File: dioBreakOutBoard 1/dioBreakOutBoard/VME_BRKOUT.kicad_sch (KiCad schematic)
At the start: 2 parts, among them J11 56509455, J12 56509455

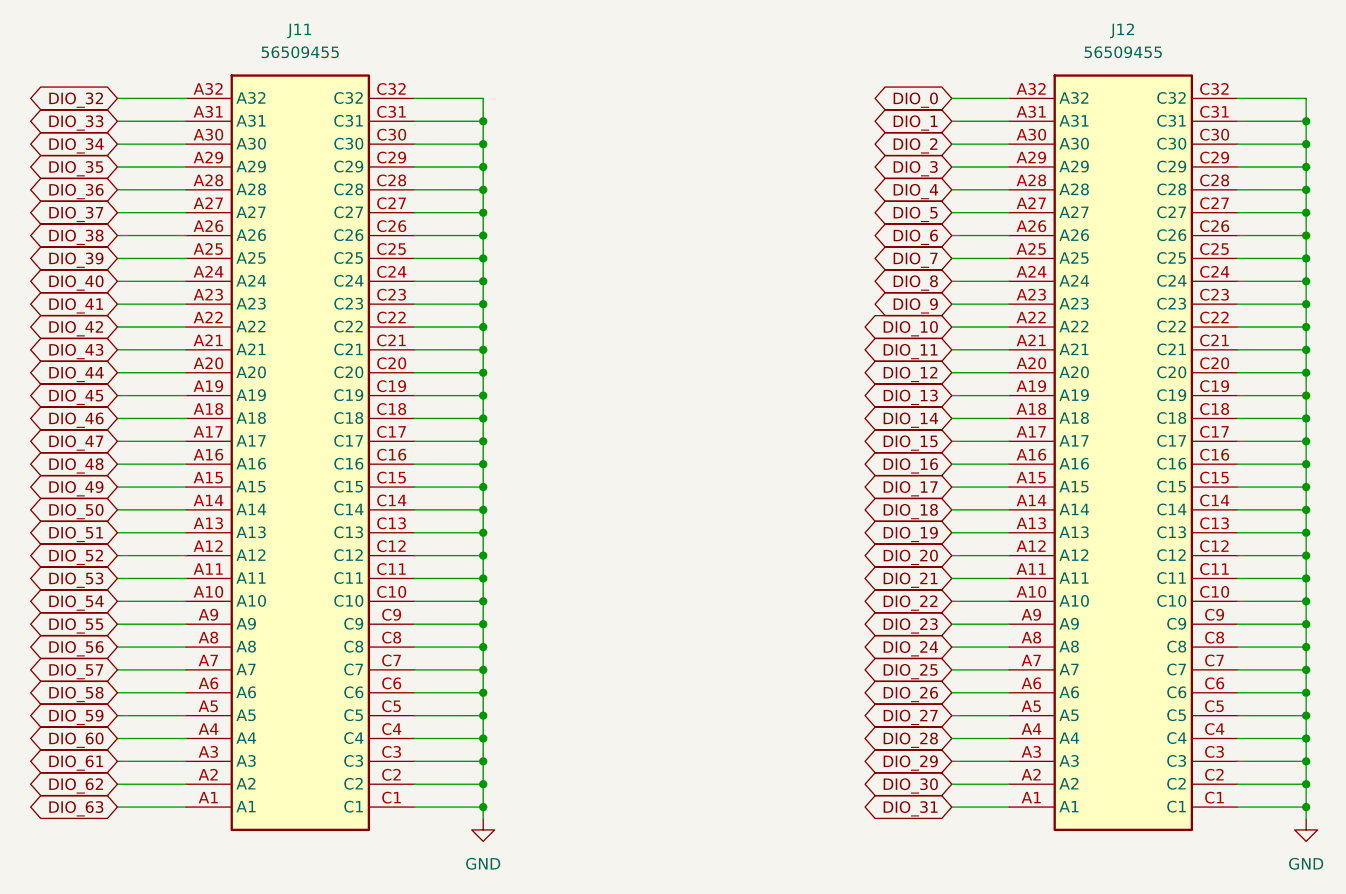
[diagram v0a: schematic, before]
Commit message: C:\Users\khernandez\KiCad\KiCad-Projects# Please enter the commit message for your changes. Lines starting
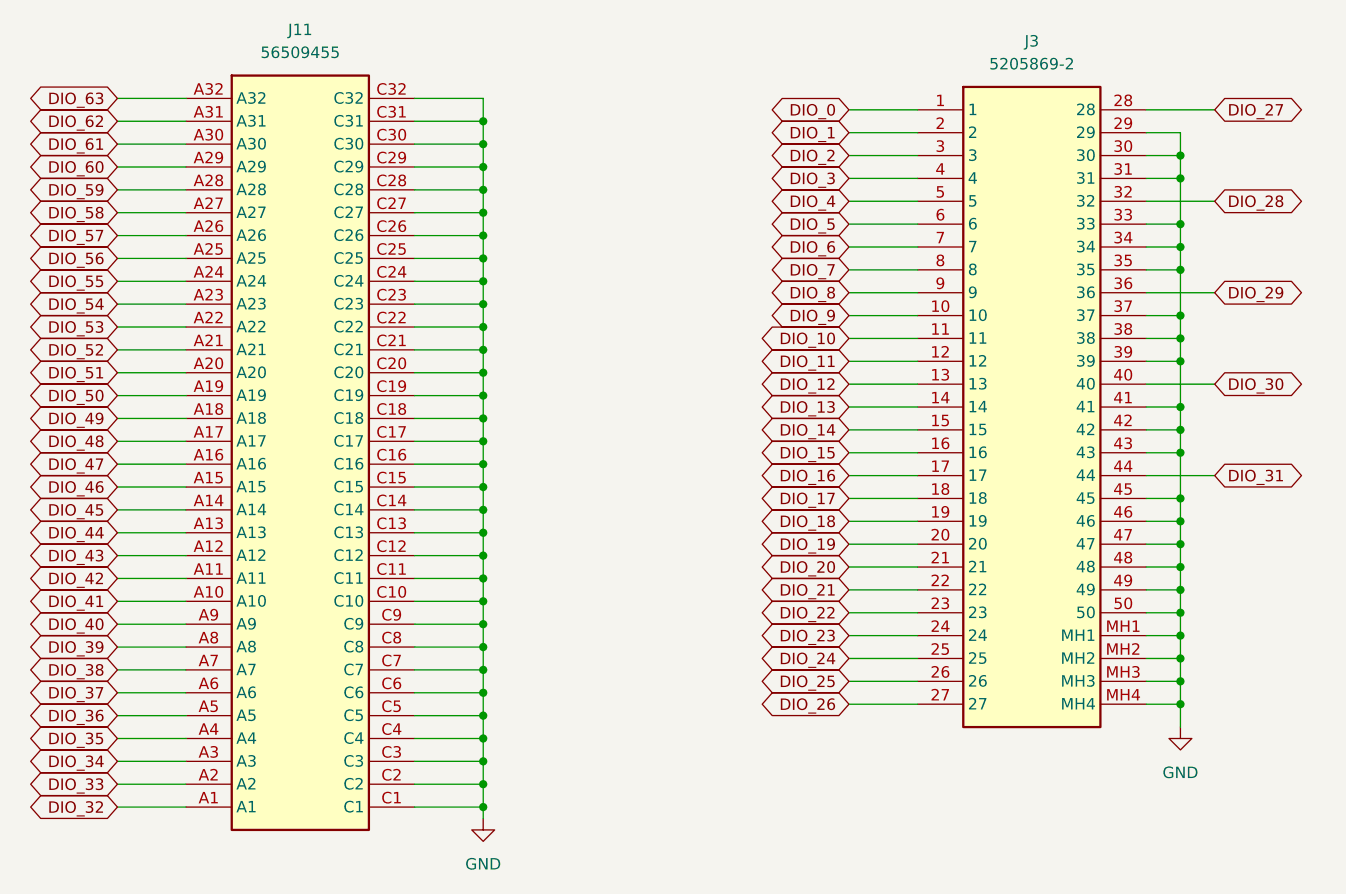
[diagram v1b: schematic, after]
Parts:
- removed J12: 56509455, Connectors_kmh:56509455, symbol 09031646922:09031646922
- added J3: 5205869-2, Connectors_kmh:52058692, symbol 5205869-2:5205869-2
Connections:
- net DIO_0: now also J3.1
- net DIO_1: now also J3.2
- net DIO_10: now also J3.11
- net DIO_11: now also J3.12
- net DIO_12: now also J3.13
- net DIO_13: now also J3.14
- net DIO_14: now also J3.15
- net DIO_15: now also J3.16
- net DIO_16: now also J3.17
- net DIO_17: now also J3.18
- net DIO_18: now also J3.19
- net DIO_19: now also J3.20
- net DIO_2: now also J3.3
- net DIO_20: now also J3.21
- net DIO_21: now also J3.22
- net DIO_22: now also J3.23
- net DIO_23: now also J3.24
- net DIO_24: now also J3.25
- net DIO_25: now also J3.26
- net DIO_26: now also J3.27
- net DIO_27: now also J3.28
- net DIO_28: now also J3.32
- net DIO_29: now also J3.36
- net DIO_3: now also J3.4
- net DIO_30: now also J3.40
- net DIO_31: now also J3.44
- net DIO_32: now also J11.A1; no longer J11.A32
- net DIO_33: now also J11.A2; no longer J11.A31
- net DIO_34: now also J11.A3; no longer J11.A30
- net DIO_35: now also J11.A4; no longer J11.A29
- net DIO_36: now also J11.A5; no longer J11.A28
- net DIO_37: now also J11.A6; no longer J11.A27
- net DIO_38: now also J11.A7; no longer J11.A26
- net DIO_39: now also J11.A8; no longer J11.A25
- net DIO_4: now also J3.5
- net DIO_40: now also J11.A9; no longer J11.A24
- net DIO_41: now also J11.A10; no longer J11.A23
- net DIO_42: now also J11.A11; no longer J11.A22
- net DIO_43: now also J11.A12; no longer J11.A21
- net DIO_44: now also J11.A13; no longer J11.A20
- net DIO_45: now also J11.A14; no longer J11.A19
- net DIO_46: now also J11.A15; no longer J11.A18
- net DIO_47: now also J11.A16; no longer J11.A17
- net DIO_48: now also J11.A17; no longer J11.A16
- net DIO_49: now also J11.A18; no longer J11.A15
- net DIO_5: now also J3.6
- net DIO_50: now also J11.A19; no longer J11.A14
- net DIO_51: now also J11.A20; no longer J11.A13
- net DIO_52: now also J11.A21; no longer J11.A12
- net DIO_53: now also J11.A22; no longer J11.A11
- net DIO_54: now also J11.A23; no longer J11.A10
- net DIO_55: now also J11.A24; no longer J11.A9
- net DIO_56: now also J11.A25; no longer J11.A8
- net DIO_57: now also J11.A26; no longer J11.A7
- net DIO_58: now also J11.A27; no longer J11.A6
- net DIO_59: now also J11.A28; no longer J11.A5
- net DIO_6: now also J3.7
- net DIO_60: now also J11.A29; no longer J11.A4
- net DIO_61: now also J11.A30; no longer J11.A3
- net DIO_62: now also J11.A31; no longer J11.A2
- net DIO_63: now also J11.A32; no longer J11.A1
- net DIO_7: now also J3.8
- net DIO_8: now also J3.9
- net DIO_9: now also J3.10
- net GND: now also J3.29, J3.30, J3.31, J3.33, J3.34, J3.35, J3.37, J3.38, J3.39, J3.41, J3.42, J3.43, J3.45, J3.46, J3.47, J3.48, J3.49, J3.50, J3.MH1, J3.MH2, J3.MH3, J3.MH4
